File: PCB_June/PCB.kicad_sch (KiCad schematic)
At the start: 26 parts, among them J2 FH34SRJ-24S-0.5SH_99_, J9 61302421121, Q1 BSS138, Q2 S8050, U3 AO3401

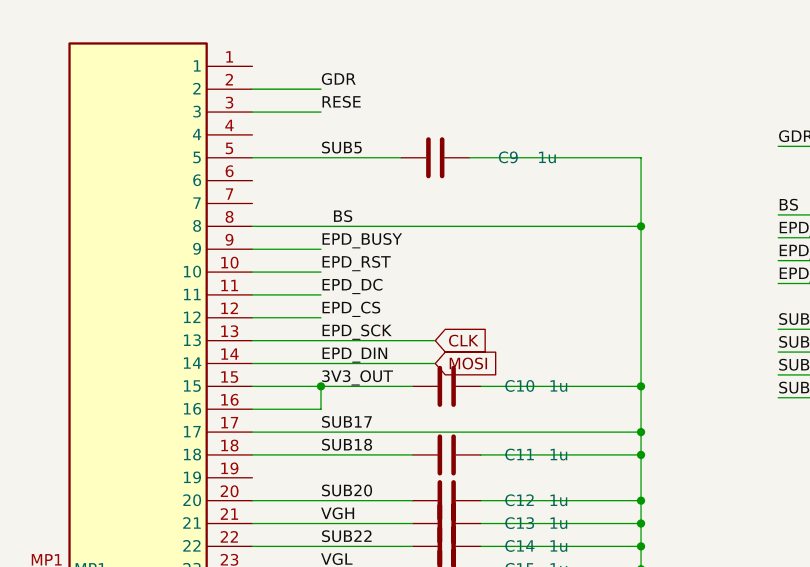
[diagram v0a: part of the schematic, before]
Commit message: yur
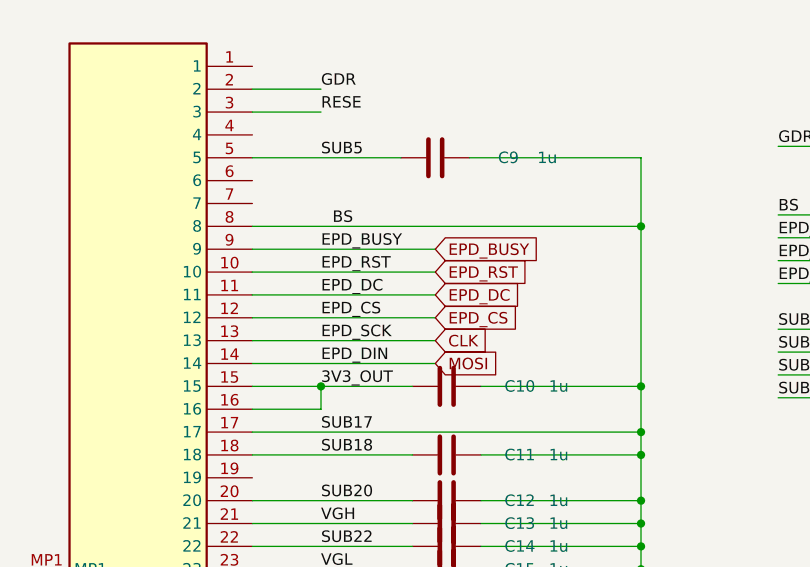
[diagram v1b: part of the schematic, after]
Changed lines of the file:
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@@
 	(wire
 		(pts
-			(xy 53.34 130.81) (xy 60.96 130.81)
+			(xy 53.34 130.81) (xy 73.66 130.81)
 		)
 		(stroke
@@
 	(wire
 		(pts
-			(xy 53.34 128.27) (xy 60.96 128.27)
+			(xy 53.34 128.27) (xy 73.66 128.27)
 		)
 		(stroke
@@
 	(wire
 		(pts
-			(xy 53.34 123.19) (xy 60.96 123.19)
+			(xy 53.34 123.19) (xy 73.66 123.19)
 		)
 		(stroke
@@
 	(wire
 		(pts
-			(xy 53.34 125.73) (xy 60.96 125.73)
+			(xy 53.34 125.73) (xy 73.66 125.73)
 		)
 		(stroke
@@
 			)
 			(justify left bottom)
+		)
+	)
+	(global_label "EPD_CS"
+		(shape input)
+		(at 73.66 130.81 0)
+		(fields_autoplaced yes)
+		(effects
+			(font
+				(size 1.27 1.27)
+			)
+			(justify left)
+		)
+		(property "Intersheetrefs" "${INTERSHEET_REFS}"
+			(at 83.7813 130.81 0)
+			(effects
+				(font
+					(size 1.27 1.27)
+				)
+				(justify left)
+				(hide yes)
+			)
+		)
+	)
+	(global_label "EPD_BUSY"
+		(shape input)
+		(at 73.66 123.19 0)
+		(fields_autoplaced yes)
+		(effects
+			(font
+				(size 1.27 1.27)
+			)
+			(justify left)
+		)
+		(property "Intersheetrefs" "${INTERSHEET_REFS}"
+			(at 86.2004 123.19 0)
+			(effects
+				(font
+					(size 1.27 1.27)
+				)
+				(justify left)
+				(hide yes)
+			)
 		)
 	)
@@
 			(effects
 				(font
+					(size 1.27 1.27)
+				)
+				(justify left)
+				(hide yes)
+			)
+		)
+	)
+	(global_label "EPD_RST"
+		(shape input)
+		(at 73.66 125.73 0)
+		(fields_autoplaced yes)
+		(effects
+			(font
+				(size 1.27 1.27)
+			)
+			(justify left)
+		)
+		(property "Intersheetrefs" "${INTERSHEET_REFS}"
+			(at 84.7489 125.73 0)
+			(effects
+				(font
+					(size 1.27 1.27)
+				)
+				(justify left)
+				(hide yes)
+			)
+		)
+	)
+	(global_label "EPD_DC"
+		(shape input)
+		(at 73.66 128.27 0)
+		(fields_autoplaced yes)
+		(effects
+			(font
+				(size 1.27 1.27)
+			)
+			(justify left)
+		)
+		(property "Intersheetrefs" "${INTERSHEET_REFS}"
+			(at 83.8418 128.27 0)
+			(effects
+				(font
